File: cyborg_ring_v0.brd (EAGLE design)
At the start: 100 x 80 mm, 44 parts, among them U1 ATTINYX5V-LEFT, U2 ATTINYX5V-RIGHT

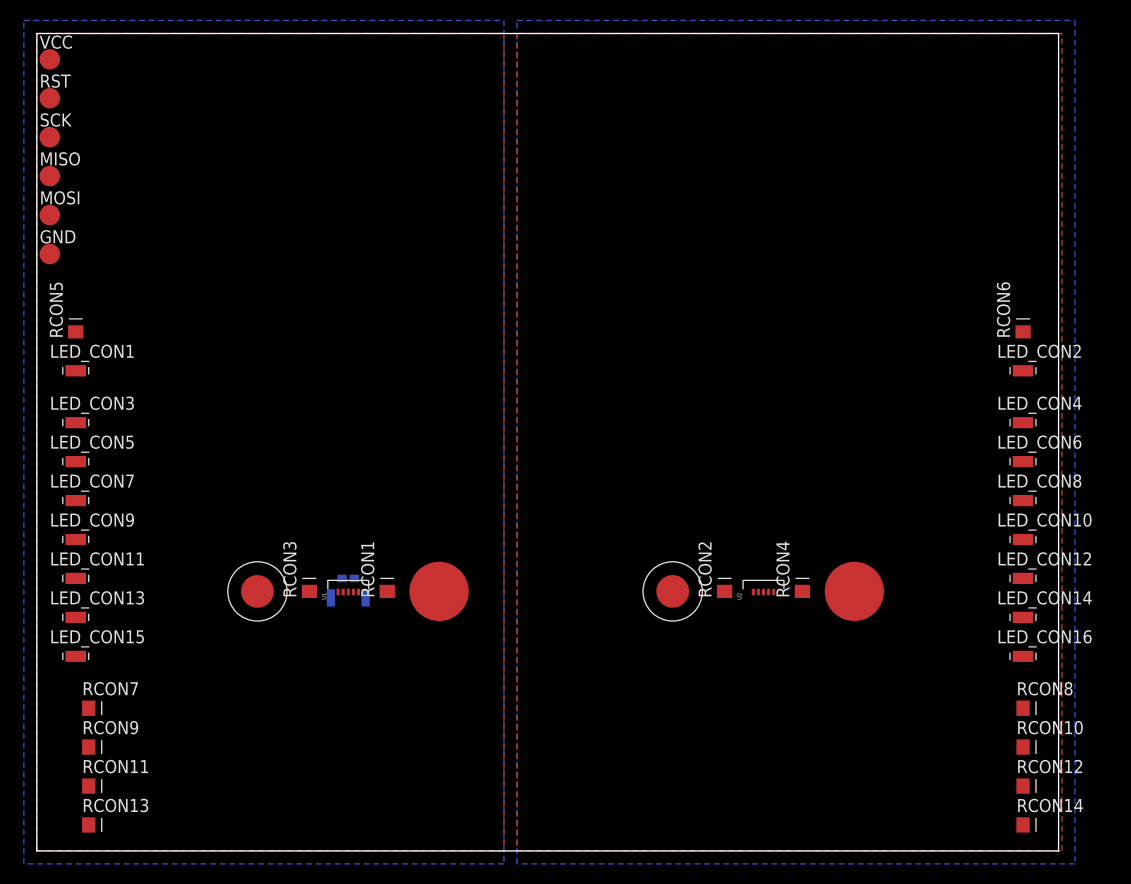
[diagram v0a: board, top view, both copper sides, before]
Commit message: Board
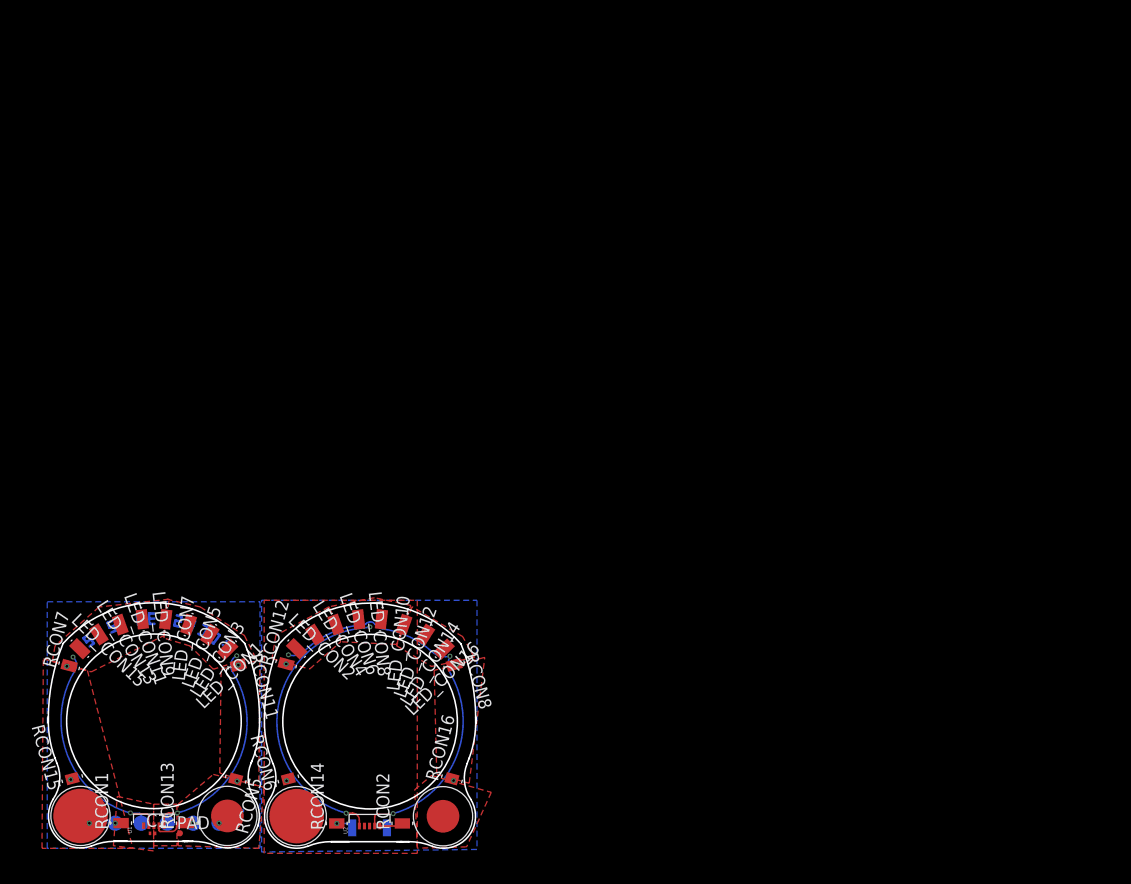
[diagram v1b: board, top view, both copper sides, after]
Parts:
- removed RCON10, RCON3, RCON4, RCON9: R0805-1/2, cyborg_ring:R0805-1/2
- added PAD: TPTP06R, testpad:TP06R
- added RCON15, RCON16: R0805-1/2TEST2, cyborg_ring:R0905-1/2BIS
- C1: device rcl:C0402K -> rcl:C0201
- GND, MISO, MOSI, RST, SCK, VCC: value TPTP20R -> TPTP15R; device testpad:TP20R -> testpad:TP15R
- RCON1, RCON11, RCON12, RCON13, RCON14, RCON2, RCON7, RCON8: value R0805-1/2 -> R0805-1/2TEST
- RCON5, RCON6: value R0805-1/2 -> R0805-1/2TEST2; device cyborg_ring:R0805-1/2 -> cyborg_ring:R0905-1/2BIS
- moved RCON6 84.2 mm to (24.6, 7.05), turned to 105 degrees
- moved LED_CON2 76.1 mm to (25.4, 19.8), turned to 315.5 degrees
- moved VCC 74.9 mm to (5.14, 2.71), flipped to the bottom
- moved RCON12 73.1 mm to (24.4, 18.3), turned to 75 degrees
- moved LED_CON4 72.3 mm to (27.2, 21.2), turned to 302.5 degrees
- moved RST 71.2 mm to (7.68, 2.71), flipped to the bottom
- moved LED_CON6 69.1 mm to (29.3, 22.2), turned to 289.5 degrees
- moved SCK 67.7 mm to (10.2, 2.71), flipped to the bottom
- moved RCON14 67.2 mm to (29.4, 2.69), turned to 90 degrees
- moved LED_CON8 66.1 mm to (31.5, 22.7), turned to 276.5 degrees
- moved MISO 64.9 mm to (15.3, 2.71), flipped to the bottom
- moved LED_CON10 63.3 mm to (33.7, 22.7), turned to 263.5 degrees
- moved LED_CON12 60.8 mm to (35.9, 22.1), turned to 250.5 degrees
- moved MOSI 60.6 mm to (12.8, 2.71), flipped to the bottom
- moved U$2 58.8 mm to (25.4, 3.40)
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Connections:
- removed net LEDL_L1: MOSI.TP
- removed net LED_L0: LED_CON1.P$1, LED_CON3.P$1, LED_CON5.P$1, LED_CON7.P$1, SCK.TP, U1.4
- removed net LED_L1: LED_CON11.P$1, LED_CON13.P$1, LED_CON15.P$1, LED_CON9.P$1, U1.1
- removed net LED_R0: LED_CON14.P$1, LED_CON16.P$1, LED_CON2.P$1, LED_CON4.P$1, U2.2
- removed net LED_R1: LED_CON10.P$1, LED_CON12.P$1, LED_CON6.P$1, LED_CON8.P$1, U2.5
- removed net N$11: U$2.P$1, U$3.P$1
- removed net SWITCH: MISO.TP, SW1.P$1, U1.2
- new net MISO/SW: MISO.TP, RCON13.1, U1.4
- new net MOSI/L1: LED_CON1.P$1, LED_CON3.P$1, LED_CON5.P$1, LED_CON7.P$1, MOSI.TP, U1.5
- new net R0: LED_CON14.P$1, LED_CON16.P$1, LED_CON2.P$1, LED_CON4.P$1, U2.4
- new net R1: LED_CON10.P$1, LED_CON12.P$1, LED_CON6.P$1, LED_CON8.P$1, U2.1
- new net SCK/L0: LED_CON11.P$1, LED_CON13.P$1, LED_CON15.P$1, LED_CON9.P$1, SCK.TP, U1.2
- new net SWITCH1: RCON14.1, SW1.P$2
- new net VCC": RCON16.1, RCON8.1
- new net VCC/2: RCON6.1, U$2.P$1, U$3.P$1
- new net VCC/2": RCON5.1
- net GND: now also PAD.TP; no longer RCON13.1, RCON3.1, RCON5.1, RCON7.1, RCON9.1, SW1.P$2
- net GND1: now also SW1.P$1; no longer RCON10.1, RCON14.1, RCON4.1, RCON6.1, RCON8.1
- net RST1: now also U2.5; no longer U2.1
- net VCC: now also RCON15.1, RCON7.1, U1.1; no longer U1.5
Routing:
- net R0: track 0.00 -> 36.6 mm, vias 0 -> 3
- net SCK/L0: track 0.00 -> 21.1 mm, vias 0 -> 2
- net R1: track 0.00 -> 21.0 mm, vias 0 -> 2
- net MOSI/L1: track 0.00 -> 20.6 mm, vias 0 -> 2
- net MISO/SW: track 0.00 -> 4.32 mm, vias 0 -> 1
- net N$20: track 0.00 -> 3.05 mm
- net N$23: track 0.00 -> 2.54 mm
- net N$13: track 0.00 -> 2.54 mm
- net N$16: track 0.00 -> 2.54 mm
- net N$18: track 0.00 -> 2.54 mm
- net RST1: track 0.00 -> 2.47 mm
- net N$22: track 0.00 -> 2.45 mm
- net N$21: track 0.00 -> 2.03 mm
- net N$3: track 0.00 -> 2.03 mm
- net N$2: track 0.00 -> 2.03 mm
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- added copper zone on layer 1, net MOSI/L1
- added copper zone on layer 1, net R0
- added copper zone on layer 1, net R1
- added copper zone on layer 1, net SCK/L0
- added copper zone on layer 1, net VCC"
- added copper zone on layer 1, net VCC
- added copper zone on layer 1, net VCC/2"
- added copper zone on layer 1, net VCC/2
- removed copper zone on layer 1, net GND1
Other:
- board size 100 x 80 mm -> 41.8 x 24 mm
